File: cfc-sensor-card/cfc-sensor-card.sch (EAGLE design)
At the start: 146 parts, among them J2 J-SAMTEC-TFM-110-X1-XXX-D-RA, J4 TFM-120-01-L-D-RA, Q1 MOSFET-PCH-SOT23-6, Q2 PMV45EN, Q3 DMP2240UDM, Q4 PMV45EN, Q5 MOSFET-PCH-SOT23-6, Q6 MOSFET-PCH-SOT23-6, Q7 MOSFET-PCH-SOT23-6, Q8 PMV45EN, U1 PIRT1280A1-12, U12 MIC842LYC5, U13 MIC842LYC5, U14 MAX4211FETE, U16 MAX7310ATE, U2 LT3042IMSE#TRPBF, U3 LT3042IMSE#TRPBF, U4 LT3042IMSE#TRPBF, U5 LT3042IMSE#TRPBF, U6 LT3042IMSE#TRPBF, U7 TLC3704IPWRPW14-M, U8 LP2985AIM5-3.3_NOPB, X1 16MHz

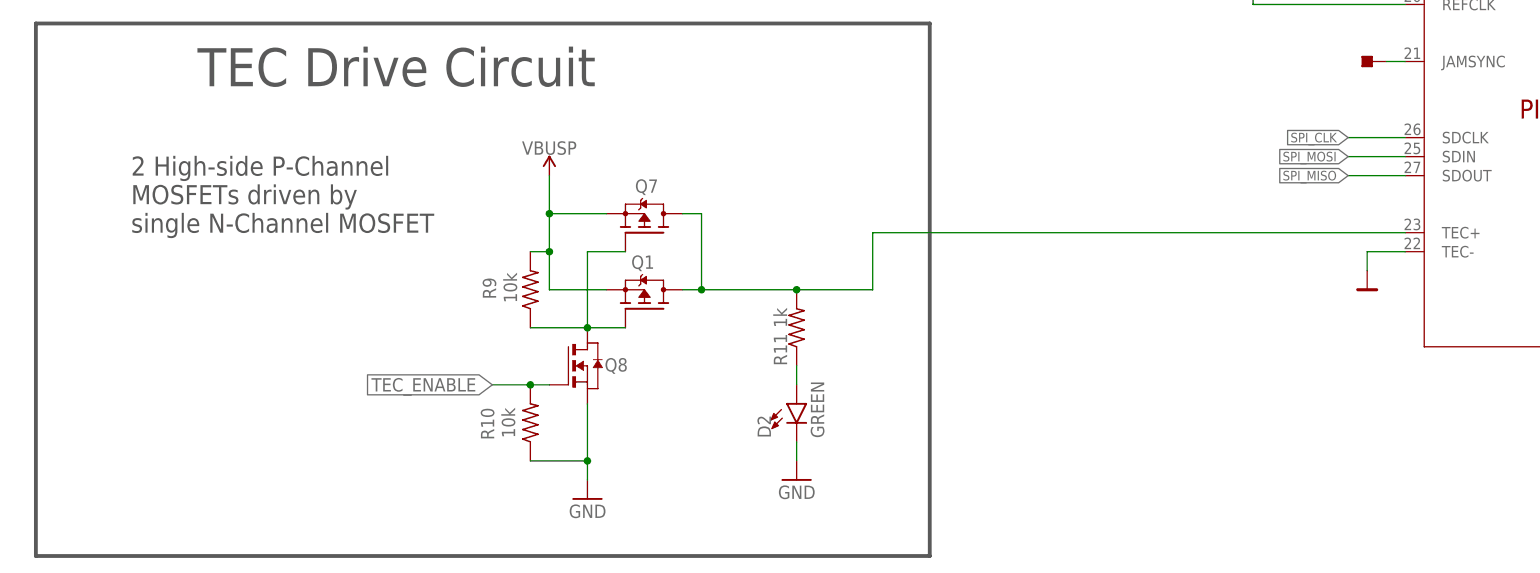
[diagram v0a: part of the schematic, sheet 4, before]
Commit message: mostly finished octavo card
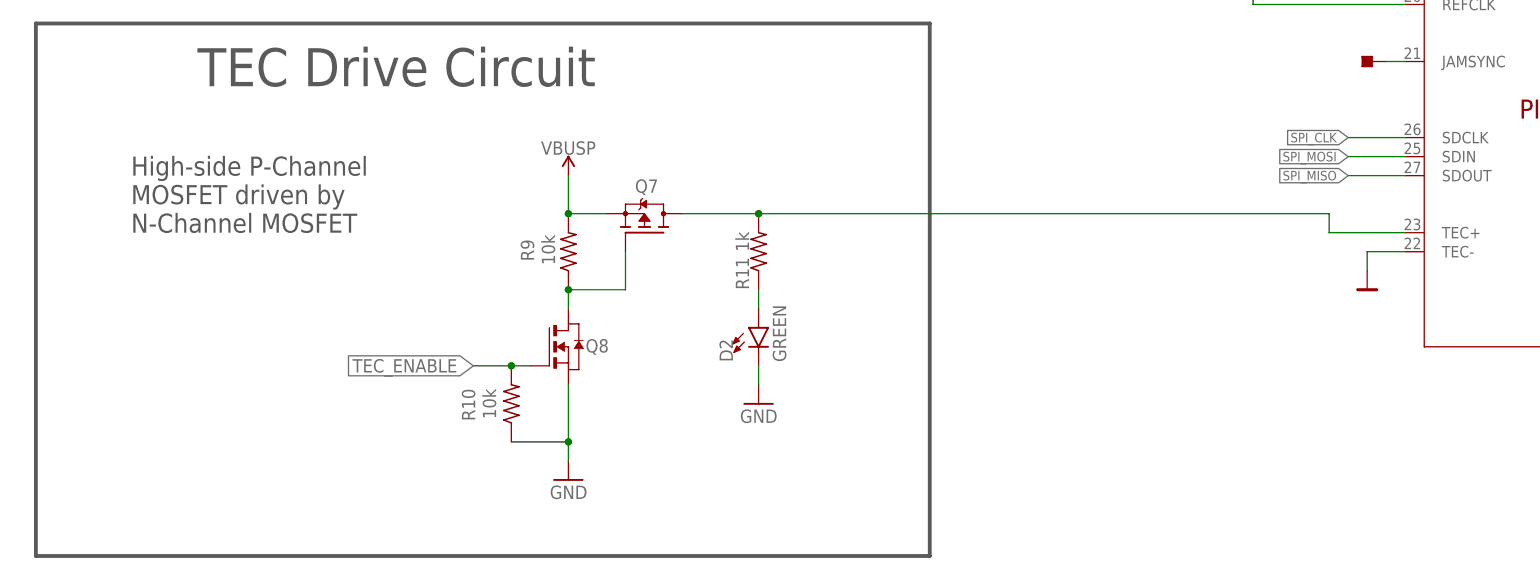
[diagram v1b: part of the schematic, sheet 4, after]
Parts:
- removed Q1: MOSFET-PCH-SOT23-6, Q-MOSFET-PCH-SOT23-6:MOSFET-PCH-SOT23-6
- R2: device R-Panasonic-EXB-2HV103JV:EXB-2HV103JV -> R-Panasonic-EXB-2HV103JV:EXB-2HV103JV-LEGACY
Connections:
- net N$3: no longer Q1.G
- net TEC+: no longer Q1.D
- net VBUSP: no longer Q1.S
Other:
- note added: "High-side P-Channel MOSFET driven by N-Channel MOSFET"
- note removed: "2 High-side P-Channel MOSFETs driven by single N-Channel MOSFET"
- moved on the sheet: D2, Q8, R10, R11, R9
